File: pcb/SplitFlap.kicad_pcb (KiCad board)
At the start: 2 copper layers, 35 x 35 mm, 23 parts, among them U1 PCF8575DBR, U2 ULN2003, U4 AP2112K-3.3

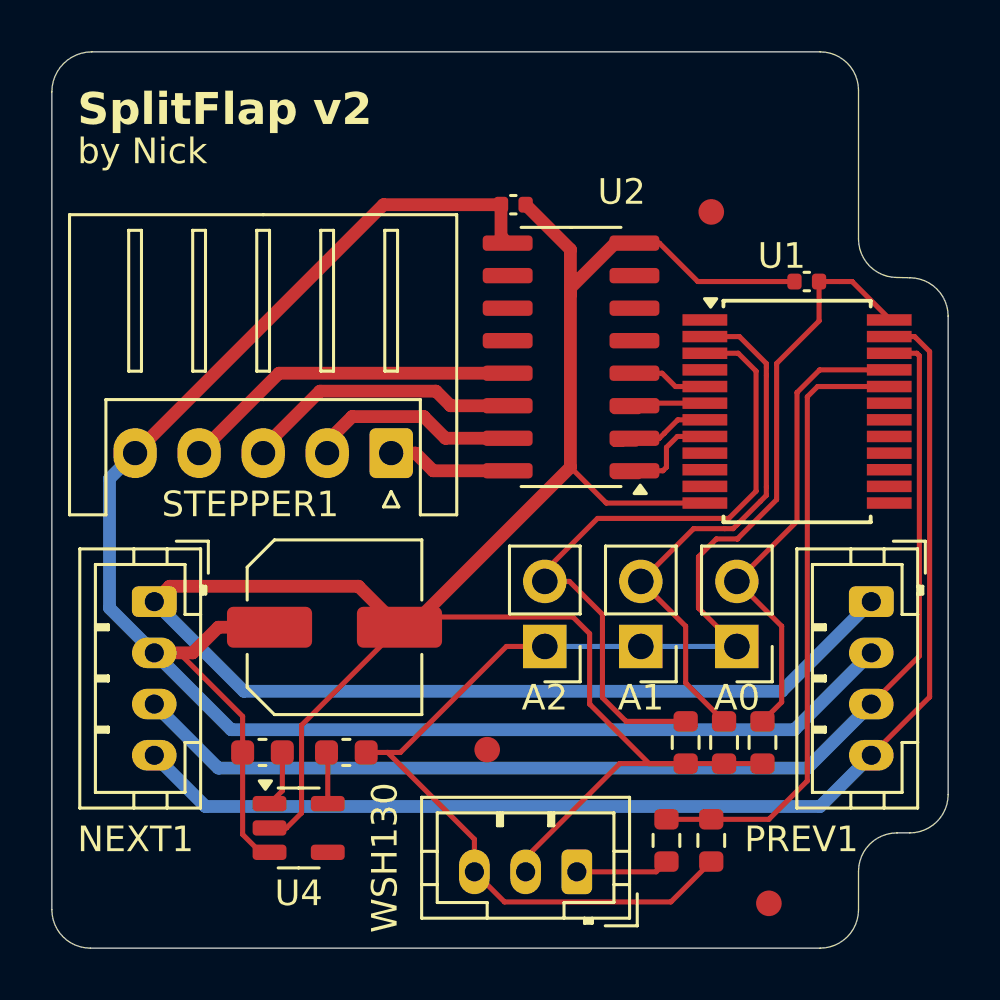
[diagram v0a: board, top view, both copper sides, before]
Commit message: Rewire PCB
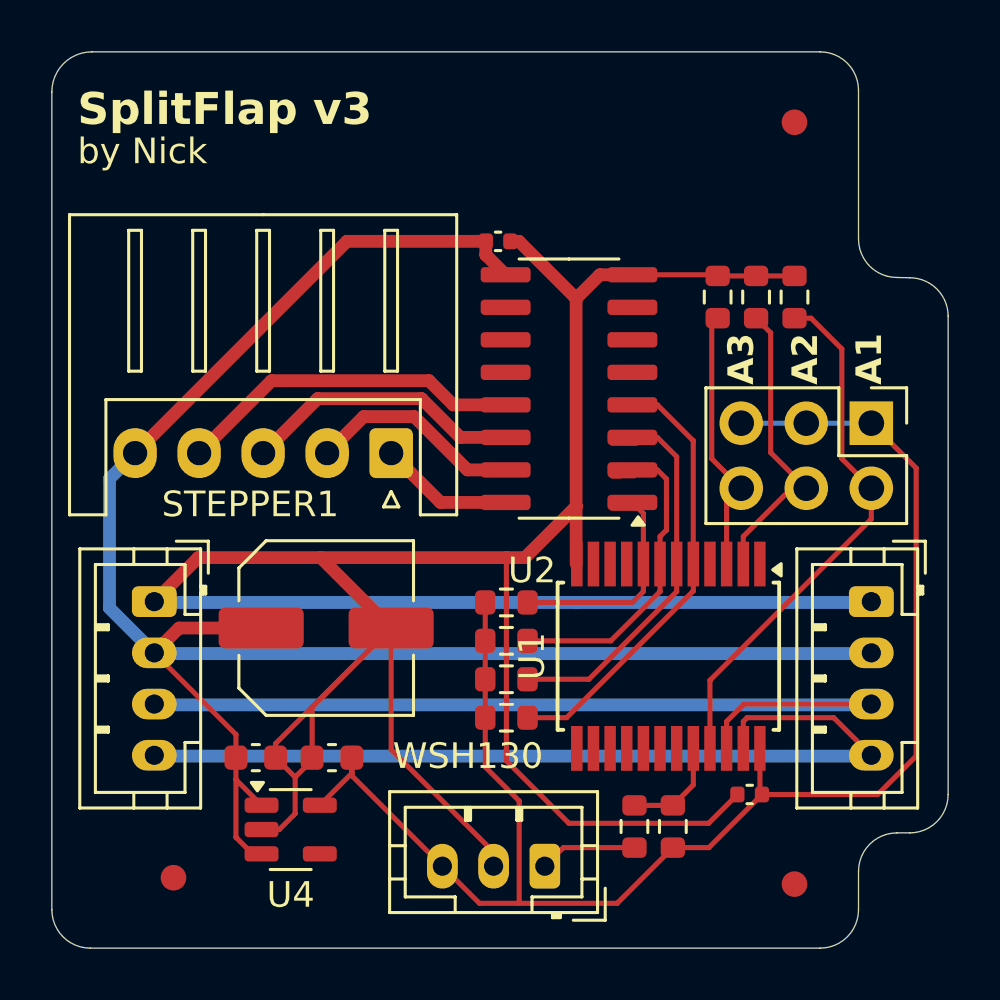
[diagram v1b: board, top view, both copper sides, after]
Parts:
- removed A0, A1, A2: Conn_01x02_Pin, Connector_PinHeader_2.54mm:PinHeader_1x02_P2.54mm_Vertical
- added J1: A1_3, Connector_PinHeader_2.54mm:PinHeader_2x03_P2.54mm_Vertical, F.Cu at (177.0, 74.0)
- added PULL_UP6: 4K7, Resistor_SMD:R_0603_1608Metric, F.Cu at (162.8, 85.5)
- added PULL_UP7: 4k7, Resistor_SMD:R_0603_1608Metric, F.Cu at (162.8, 84.0)
- added PULL_UP8: 4k7, Resistor_SMD:R_0603_1608Metric, F.Cu at (162.8, 82.5)
- added PULL_UP9: 4k7, Resistor_SMD:R_0603_1608Metric, F.Cu at (162.8, 81.0)
- moved REF** 23.3 mm to (149.8, 91.8)
- moved C1 20.2 mm to (172.2, 88.5)
- moved PULL_UP5 17.9 mm to (174.0, 69.1), turned to 90 degrees
- moved PULL_UP3 17.5 mm to (171.0, 69.1), turned to 90 degrees
- moved PULL_UP4 17.4 mm to (172.5, 69.1), turned to 90 degrees
- moved REF** 13.1 mm to (174.0, 92.0)
- moved U1 10.8 mm to (169.1, 83.1), turned to -90 degrees
- moved REF** 4.78 mm to (174.0, 62.2)
- moved PULL_UP2 1.60 mm to (169.2, 89.8)
- moved C2_BYPASS1 1.55 mm to (162.4, 66.9)
- moved SERIES1 1.36 mm to (167.8, 89.8)
- moved WSH130 1.27 mm to (164.2, 91.3)
- moved U2 1.24 mm to (165.2, 72.7)
- moved C3 0.60 mm to (155.9, 87.1)
- moved C2 0.33 mm to (153.0, 87.1), turned to 180 degrees
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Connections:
- C2 pad 1: +5V -> GND
- C2 pad 2: Net-(U4-VIN) -> +5V
- C3 pad 1: Net-(U4-VOUT) -> GND
- PULL_UP3 pad 1: Net-(A0-Pin_2) -> Net-(J1-Pin_6)
- PULL_UP5 pad 1: Net-(A2-Pin_2) -> Net-(J1-Pin_2)
- U1 pad 21: Net-(A0-Pin_2) -> Net-(J1-Pin_2)
- U1 pad 3: Net-(A2-Pin_2) -> Net-(J1-Pin_6)
- U4 pad 1: Net-(U4-VIN) -> +5V
- U4 pad 5: Net-(U4-VOUT) -> +3.3V
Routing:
- net Net-(A2-Pin_2): track 26.2 -> 0.00 mm
- net Net-(J1-Pin_2): track 0.00 -> 21.0 mm
- net Net-(U1-P17): track 24.5 -> 4.06 mm
- net Net-(A0-Pin_2): track 18.5 -> 0.00 mm
- net Net-(U1-P1): track 2.97 -> 17.3 mm
- net Net-(NEXT1-Pin_4): track 48.2 -> 34.7 mm
- net Net-(U1-P2): track 3.76 -> 15.5 mm
- net Net-(NEXT1-Pin_3): track 45.7 -> 35.0 mm
- net Net-(J1-Pin_6): track 0.00 -> 10.4 mm
- net Net-(J1-Pin_4): track 20.7 -> 11.8 mm
- net Net-(U1-P3): track 4.27 -> 13.2 mm
- net +3.3V: track 53.7 -> 62.5 mm
- net GND: track 116.0 -> 120.6 mm
- net Net-(U1-P4): track 4.73 -> 9.33 mm
- net +5V: track 74.7 -> 71.5 mm
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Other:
- board text added: "A1"
- board text added: "A2"
- board text added: "A3"
- board text added: "SplitFlap v3"
- board text removed: "SplitFlap v2"
